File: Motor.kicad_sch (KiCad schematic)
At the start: 0 parts

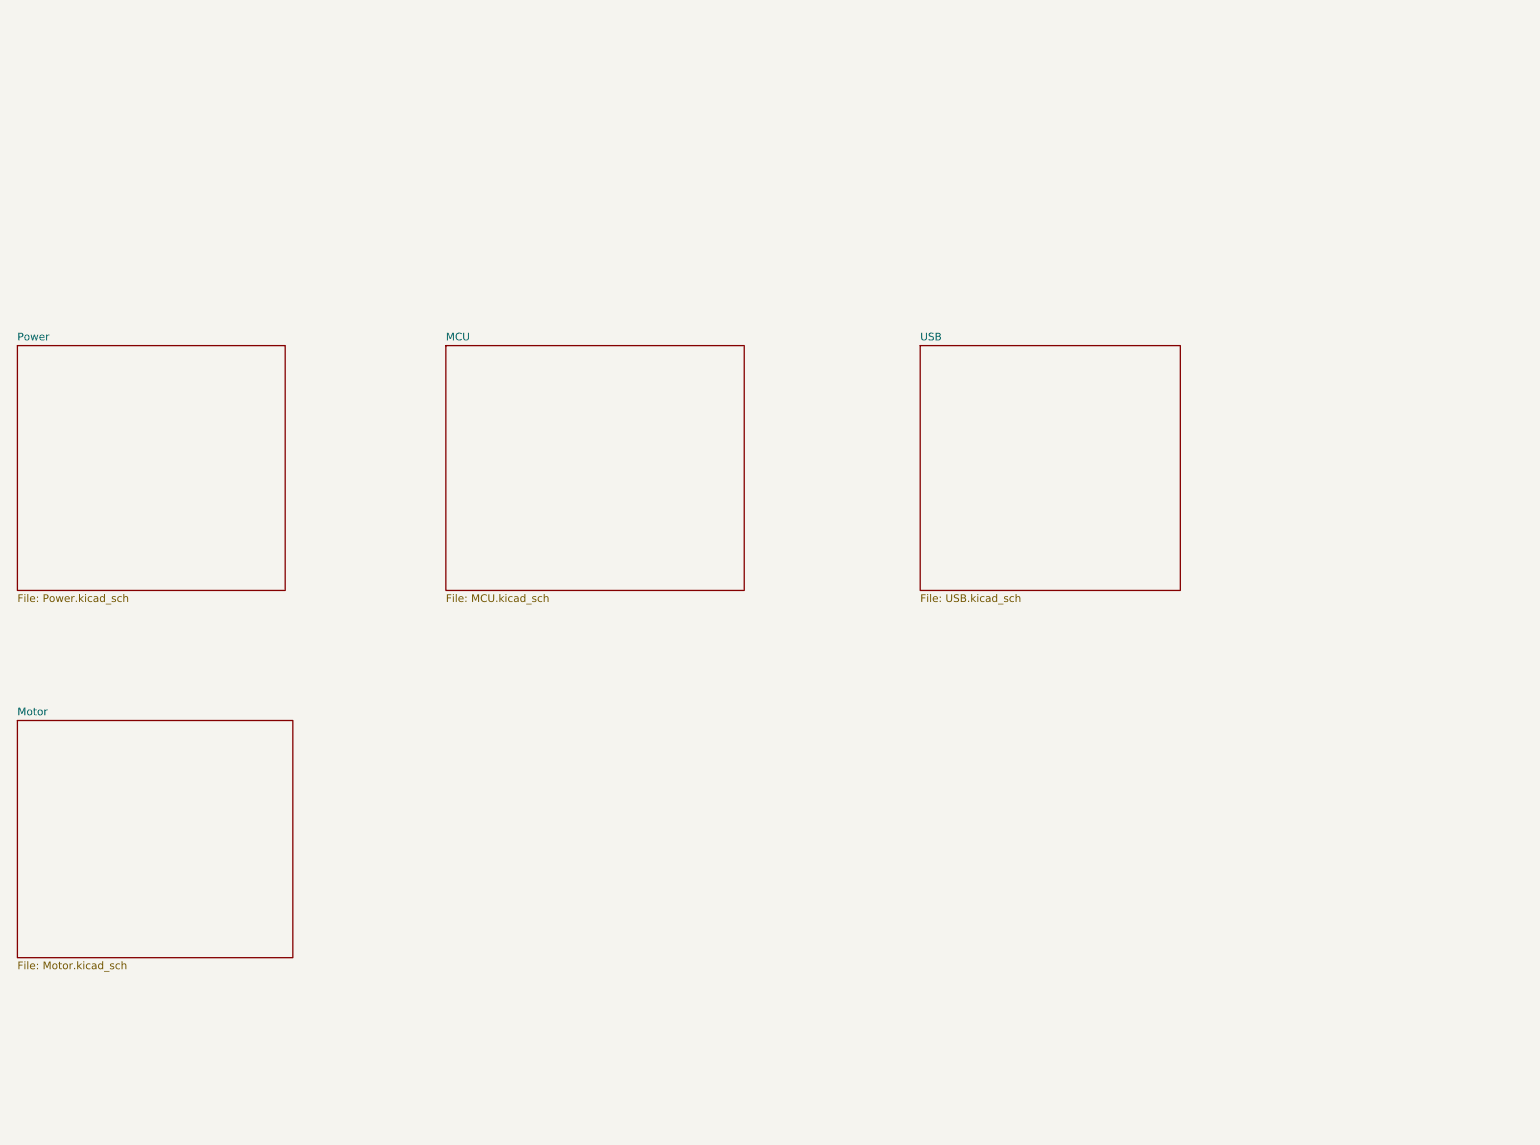
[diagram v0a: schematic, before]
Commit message: Finished Updating Schematics
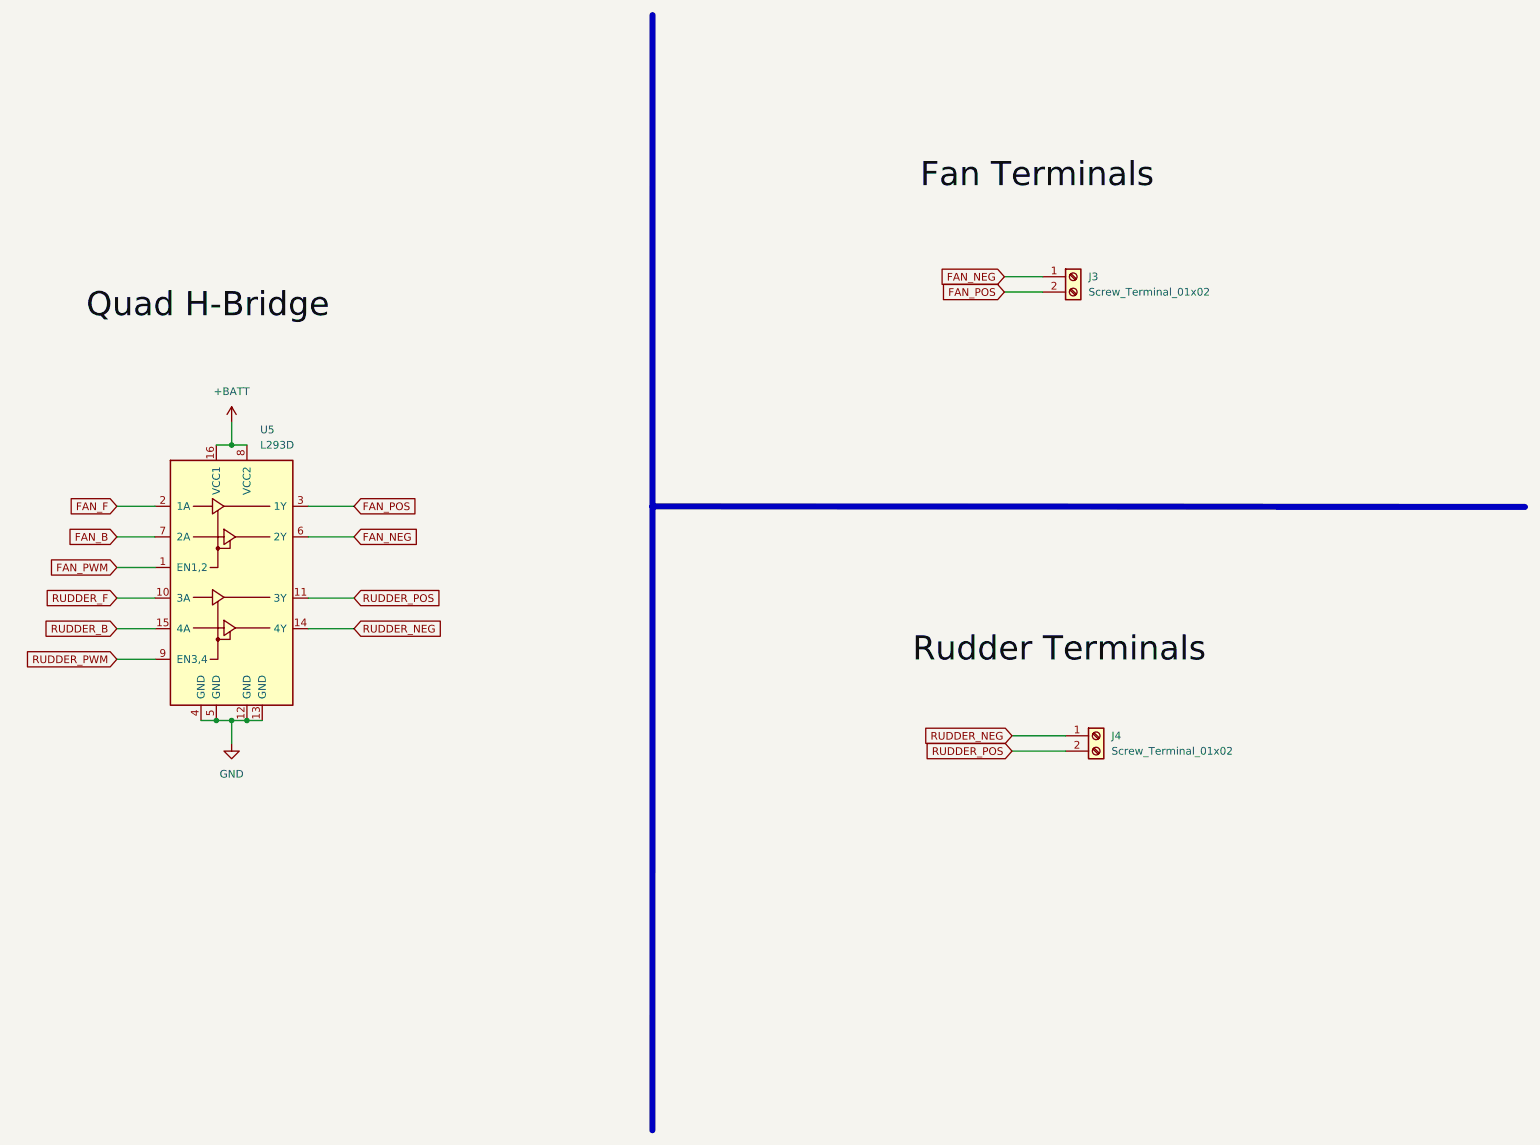
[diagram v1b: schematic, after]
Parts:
- added J3, J4: Screw_Terminal_01x02, symbol Connector:Screw_Terminal_01x02
- added U5: L293D, Package_DIP:DIP-16_W7.62mm, symbol Driver_Motor:L293D
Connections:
- new net +BATT: U5.16 (VCC1), U5.8 (VCC2)
- new net FAN_B: U5.7 (2A)
- new net FAN_F: U5.2 (1A)
- new net FAN_NEG: J3.1 (Pin_1), U5.6 (2Y)
- new net FAN_POS: J3.2 (Pin_2), U5.3 (1Y)
- new net FAN_PWM: U5.1 (EN1,2)
- new net GND: U5.12 (GND), U5.13 (GND), U5.4 (GND), U5.5 (GND)
- new net RUDDER_B: U5.15 (4A)
- new net RUDDER_F: U5.10 (3A)
- new net RUDDER_NEG: J4.1 (Pin_1), U5.14 (4Y)
- new net RUDDER_POS: J4.2 (Pin_2), U5.11 (3Y)
- new net RUDDER_PWM: U5.9 (EN3,4)
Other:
- removed sheet MCU
- removed sheet Motor
- removed sheet Power
- removed sheet USB
- company: Insight Wisconsin -> (none)
